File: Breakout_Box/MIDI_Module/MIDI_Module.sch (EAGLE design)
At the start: 71 parts, among them T1 2N2222, T2 2N2222, U1 TLV6004, U2 TLV6004, U3 MIC5205-5.0YM5-TR, U4 MIC5205-3.3YM5-TR

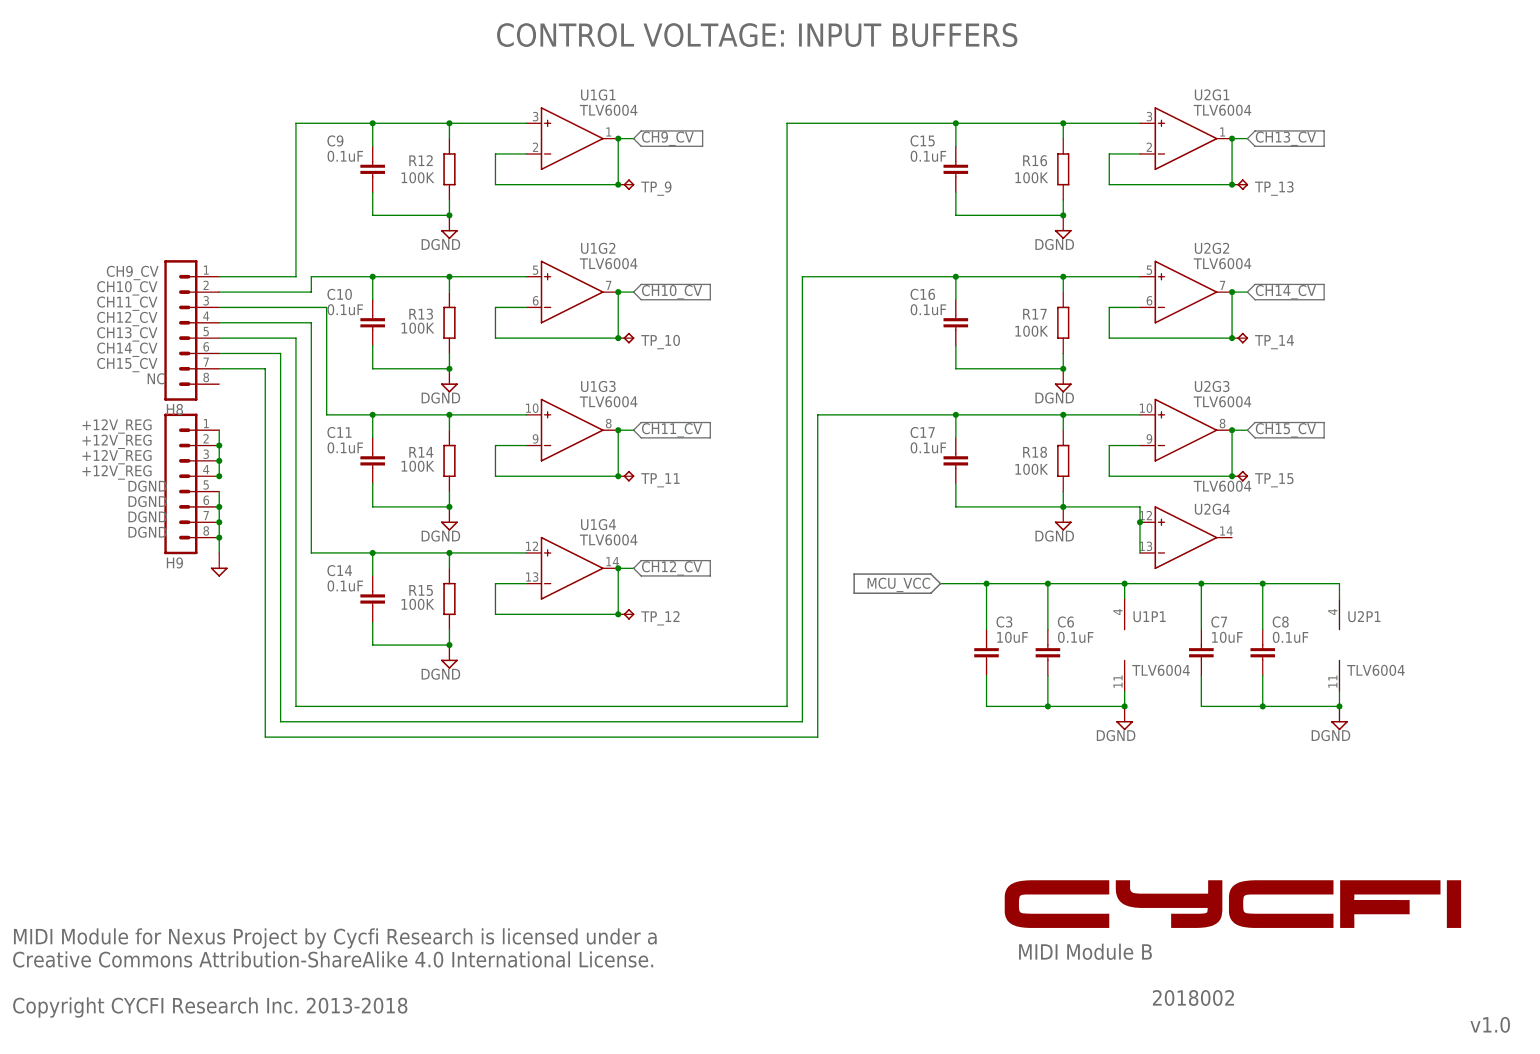
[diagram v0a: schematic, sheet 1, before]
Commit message: merge version_1.1 to devel
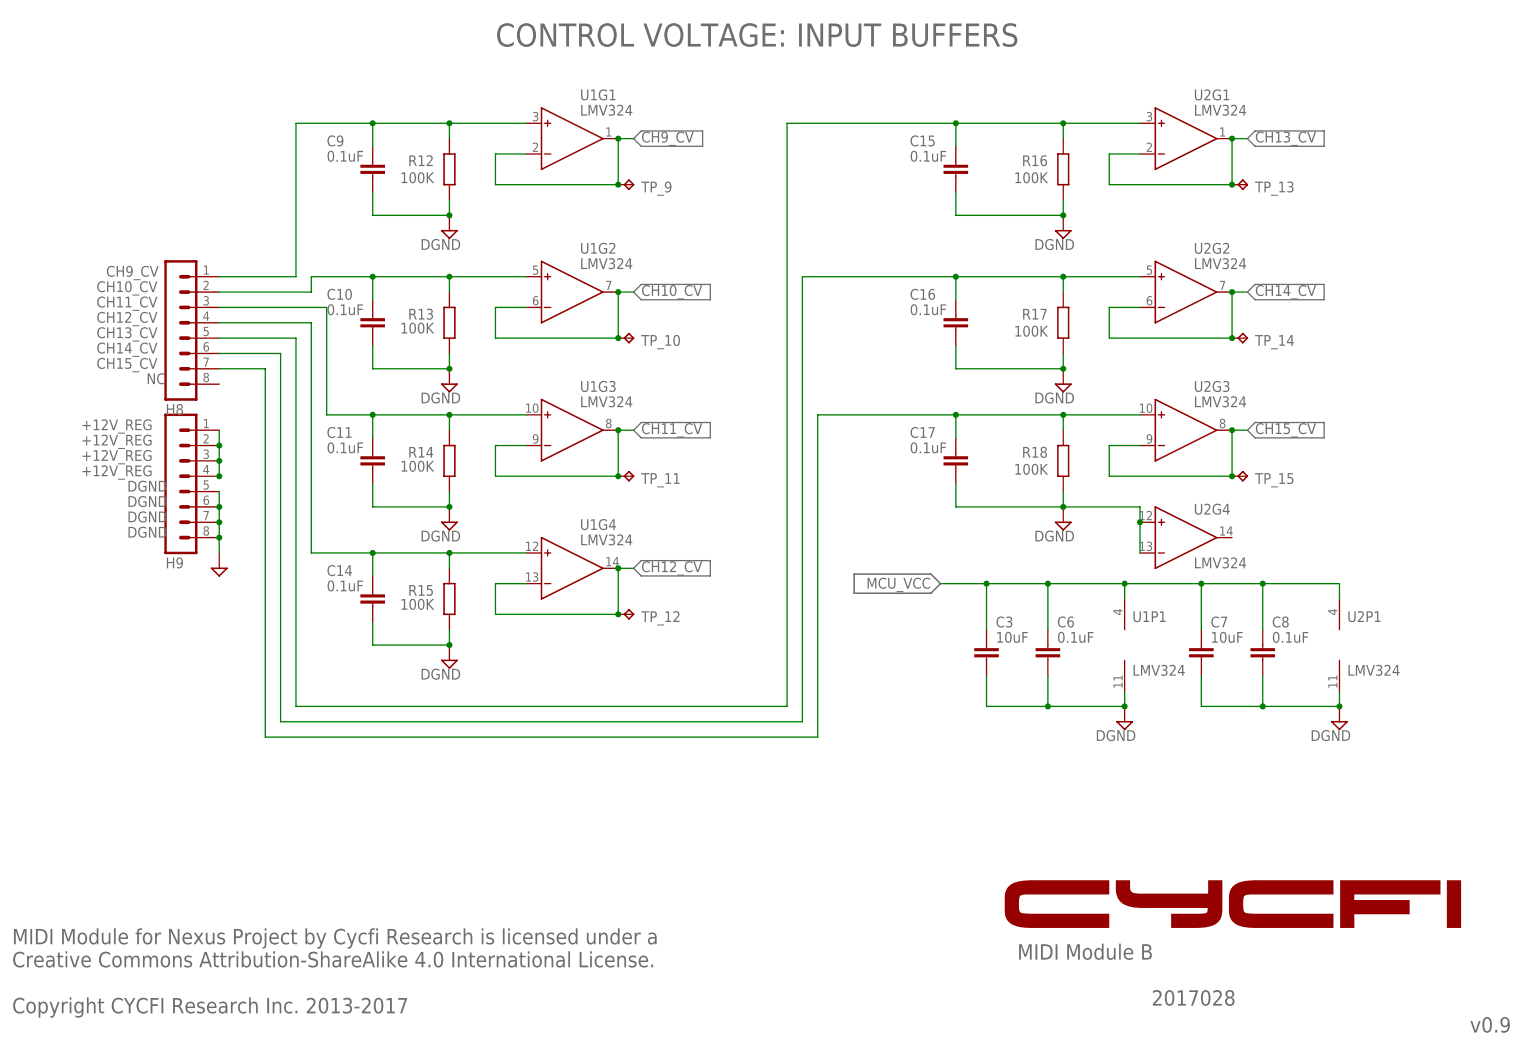
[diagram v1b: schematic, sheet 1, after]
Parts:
- U1, U2: value TLV6004 -> LMV324; device CYCFI_semicon:TLV6004 -> CYCFI_semicon:LMV324
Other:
- note added: "2017028"
- note added: "MIDI Module for Nexus Project by Cycfi Research is licensed under a Creative Commons Attribution-ShareAlike 4.0 International License. Copyright CYCFI Research Inc. 2013-2017"
- note added: "v0.9"
- note added: "v0.92"
- note removed: "2018002"
- note removed: "MIDI Module for Nexus Project by Cycfi Research is licensed under a Creative Commons Attribution-ShareAlike 4.0 International License. Copyright CYCFI Research Inc. 2013-2018"
- note removed: "v1.0"

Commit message: reset devel
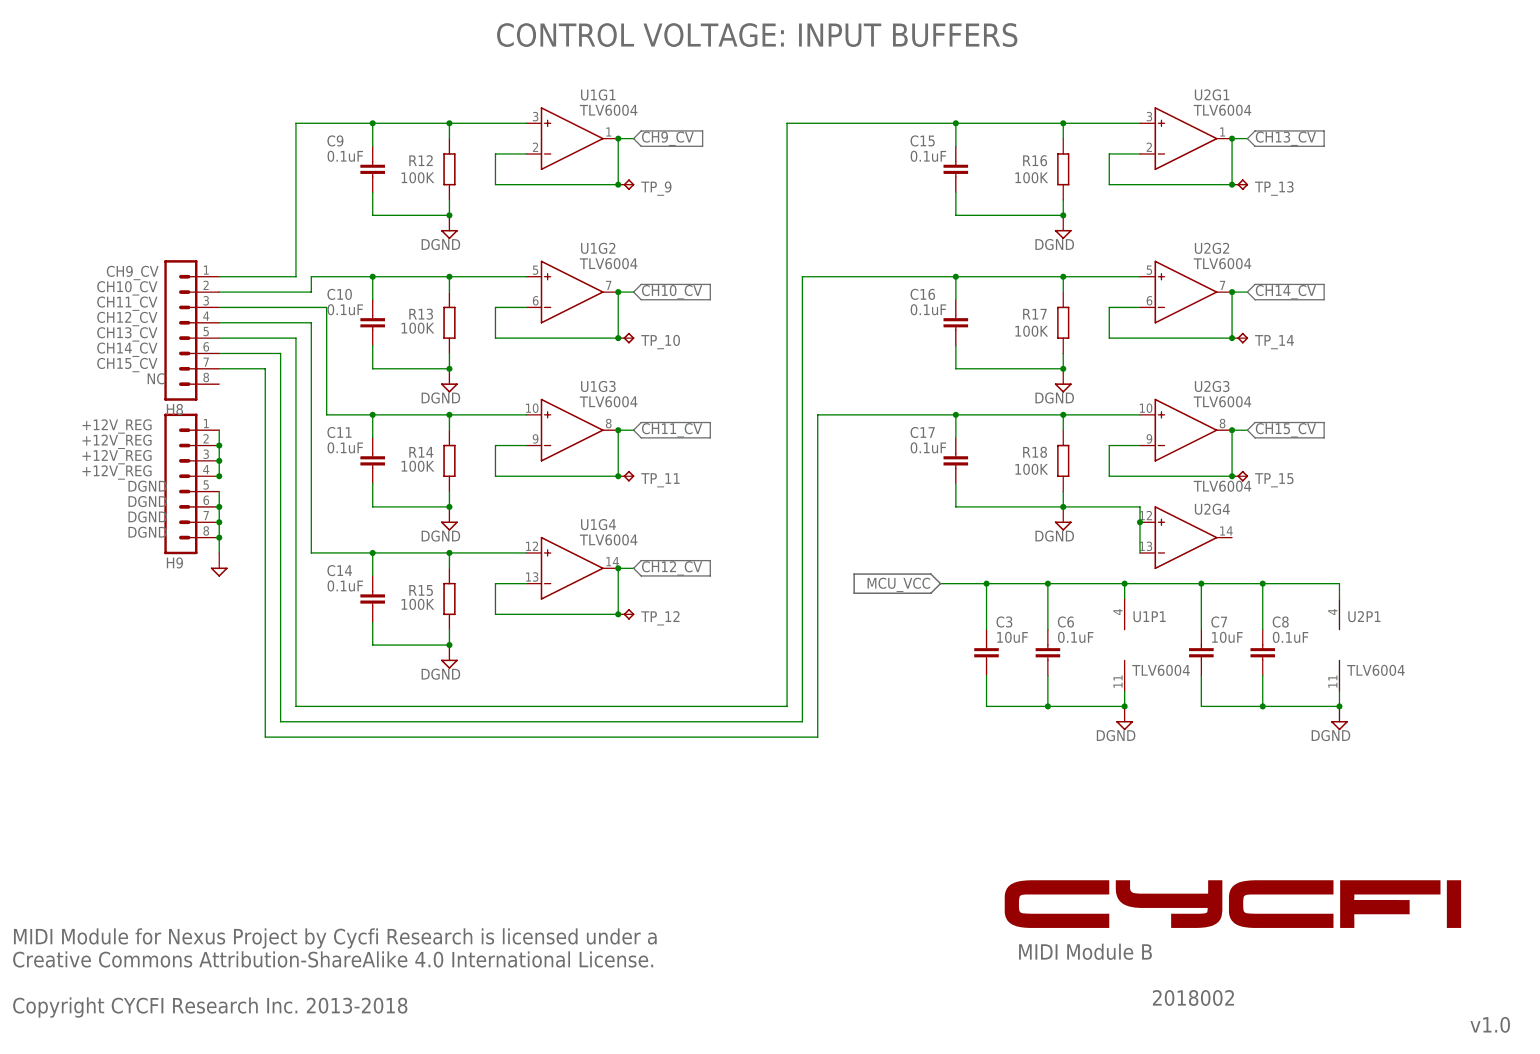
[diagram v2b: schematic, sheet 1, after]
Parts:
- U1, U2: value LMV324 -> TLV6004; device CYCFI_semicon:LMV324 -> CYCFI_semicon:TLV6004
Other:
- note added: "2018002"
- note added: "MIDI Module for Nexus Project by Cycfi Research is licensed under a Creative Commons Attribution-ShareAlike 4.0 International License. Copyright CYCFI Research Inc. 2013-2018"
- note added: "v1.0"
- note removed: "2017028"
- note removed: "MIDI Module for Nexus Project by Cycfi Research is licensed under a Creative Commons Attribution-ShareAlike 4.0 International License. Copyright CYCFI Research Inc. 2013-2017"
- note removed: "v0.9"
- note removed: "v0.92"
